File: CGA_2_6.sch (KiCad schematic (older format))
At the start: 14 parts, among them U24 74LS244, U32 74LS166, U33 27C256, U34 74LS273, U35 74LS273, U36 74LS244, U37 74LS374, U39 74LS174, U68 74LS86, U7 74LS166, U9 74153

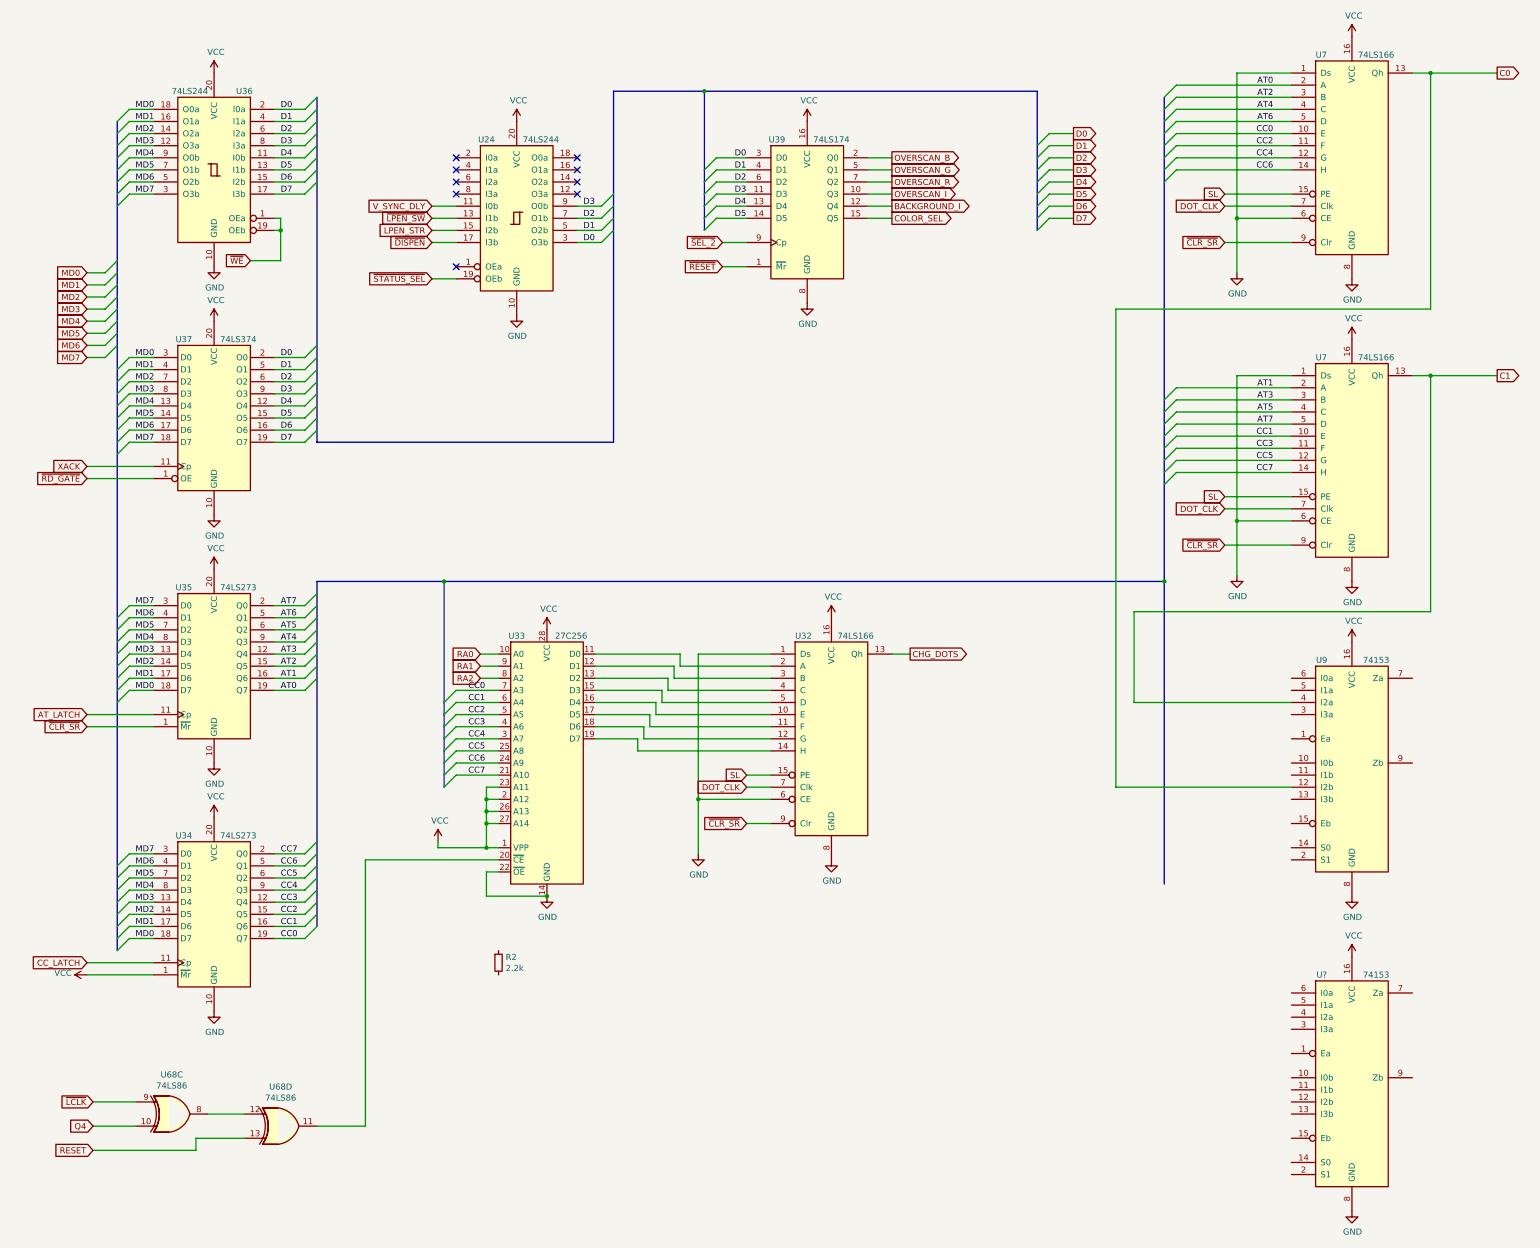
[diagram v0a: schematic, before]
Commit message: More sheet 2
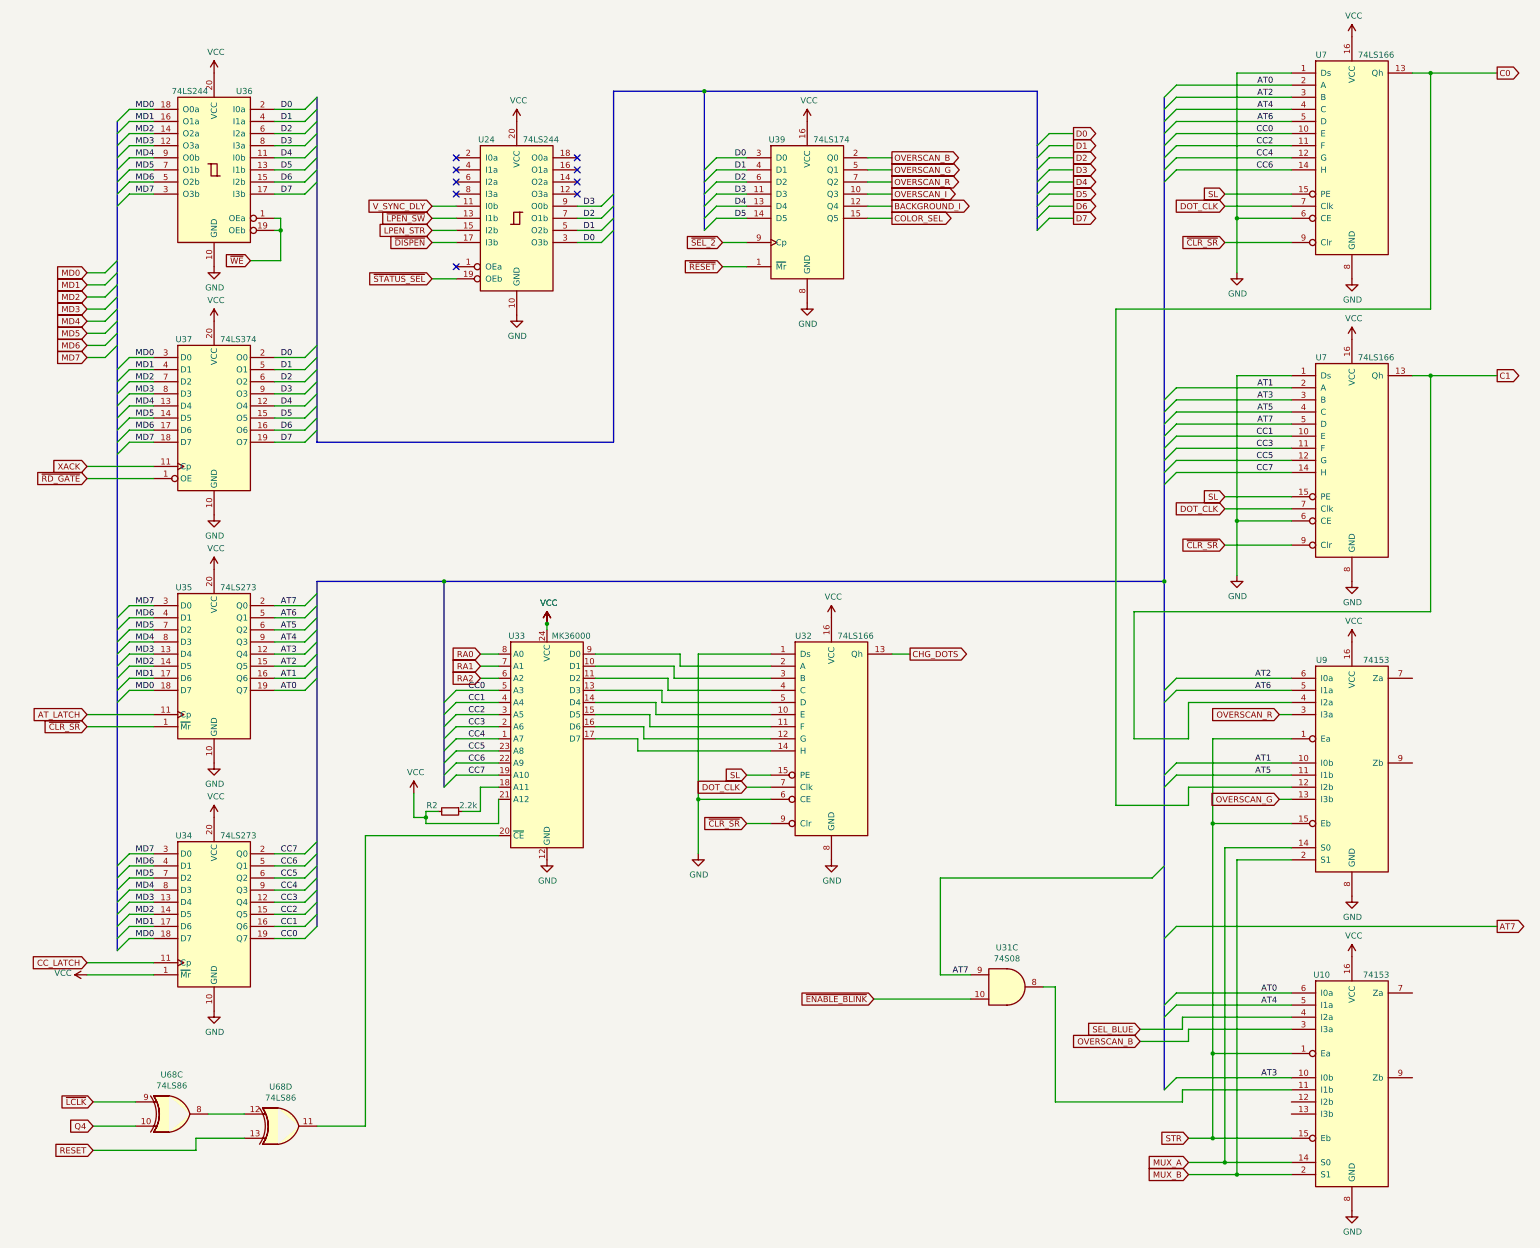
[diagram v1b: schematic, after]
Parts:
- removed U33: 27C256, Package_DIP:DIP-28_W15.24mm_LongPads, symbol Memory_EPROM:27C256
- added U31: 74S08, Package_DIP:DIP-14_W7.62mm_LongPads, symbol 74xx:74LS08
- added U33: MK36000, Package_DIP:DIP-24_W15.24mm_LongPads, symbol ISA_CGA:MK36000
- gave numbers to parts that had none: 1
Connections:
- net AT0: now also U10.6 (I0a)
- net AT1: now also U9.10 (I0b)
- net AT2: now also U9.6 (I0a)
- net AT3: now also U10.10 (I0b)
- net AT4: now also U10.5 (I1a)
- net AT5: now also U9.11 (I1b)
- net AT6: now also U9.5 (I1a)
- net AT7: now also U31.9
- net CC0: now also U33.5 (A3)
- net CC1: now also U33.4 (A4)
- net CC2: now also U33.3 (A5)
- net CC3: now also U33.2 (A6)
- net CC4: now also U33.1 (A7)
- net CC5: now also U33.23 (A8)
- net CC6: now also U33.22 (A9)
- net CC7: now also U33.19 (A10)
- net GND: now also U33.12 (GND)
- net OVERSCAN_B: now also U10.3 (I3a)
- net OVERSCAN_G: now also U9.13 (I3b)
- net OVERSCAN_R: now also U9.3 (I3a)
- net RA0: now also U33.8 (A0)
- net RA1: now also U33.7 (A1)
- net RA2: now also U33.6 (A2)
- net VCC: now also R2.2, U33.21 (A12), U33.24 (VCC)
- net at U32.2 (A): now also U33.9 (D0)
- net at U32.3 (B): now also U33.10 (D1)
- net at U32.4 (C): now also U33.11 (D2)
- net at U32.5 (D): now also U33.13 (D3)
- net at U32.10 (E): now also U33.14 (D4)
- net at U32.11 (F): now also U33.15 (D5)
- net at U32.12 (G): now also U33.16 (D6)
- net at U32.14 (H): now also U33.17 (D7)
- net at U68.11: now also U33.20 (~CE)
- net STR: now reaches U9.1 (Ea)
- net STR: now also U10.1 (Ea), U10.15 (Eb), U9.15 (Eb)
- net MUX_A: now reaches U9.14 (S0)
- net MUX_A: now also U10.14 (S0)
- net MUX_B: now reaches U9.2 (S1)
- net MUX_B: now also U10.2 (S1)
- net at U10.11 (I1b): now also U31.8
- net SEL_BLUE: now reaches U10.4 (I2a)
- net at R2.1: now also U33.18 (A11)
- new net ~ENABLE_BLINK: U31.10
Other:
- moved on the sheet: R2
